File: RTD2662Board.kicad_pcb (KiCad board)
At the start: 2 copper layers, 100 x 65 mm, 227 parts, among them J1 USB_B, J10 Conn_Coaxial, J11 Conn_01x03, J2 AudioJack4, J3 Jack, J4 Conn_02x25_Odd_Even, J5 AudioJack4, J6 DVI_FEMALE, J7 HDMI_A_1.4, J8 Mini-DIN-4, J9 DB15_Female_HighDensity_Mount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, Q5 BC846, Q7 AO3401A, Q8 BC846, Q9 BC846, SW1 SW_Push, SW2 SW_Push, SW3 SW_Push, SW4 SW_Push, SW5 SW_Push, U1 TSOP382xx, U10 TPS61040DBV, U11 TPS61040DBV, U12 CH341T, U2 ES7134S, U4 PAM8003, U5 TPS61040DBV, U6 APW7313, U7 AMS1117-1.8, U8 RTD2662, U9 W25Qxx, Y1 Crystal, Y2 Crystal

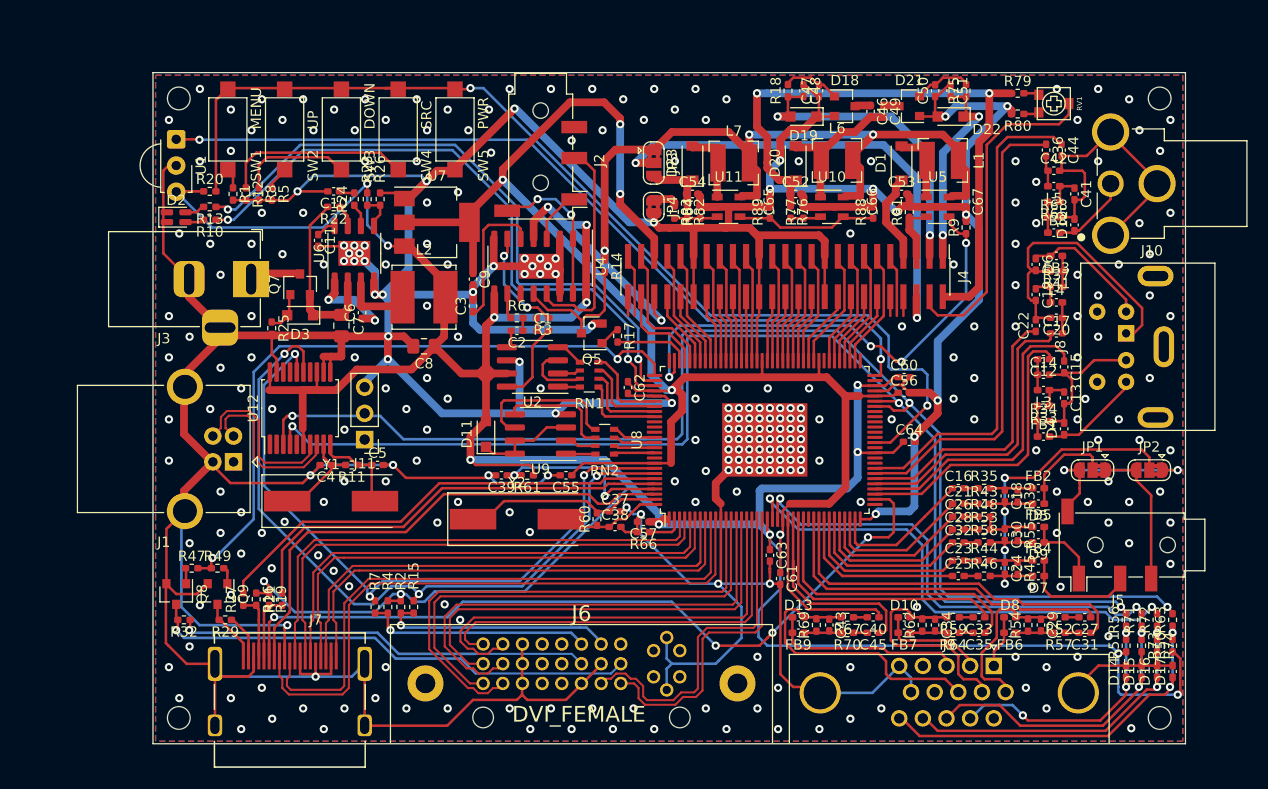
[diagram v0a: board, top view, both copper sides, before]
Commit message: Revision 0.2
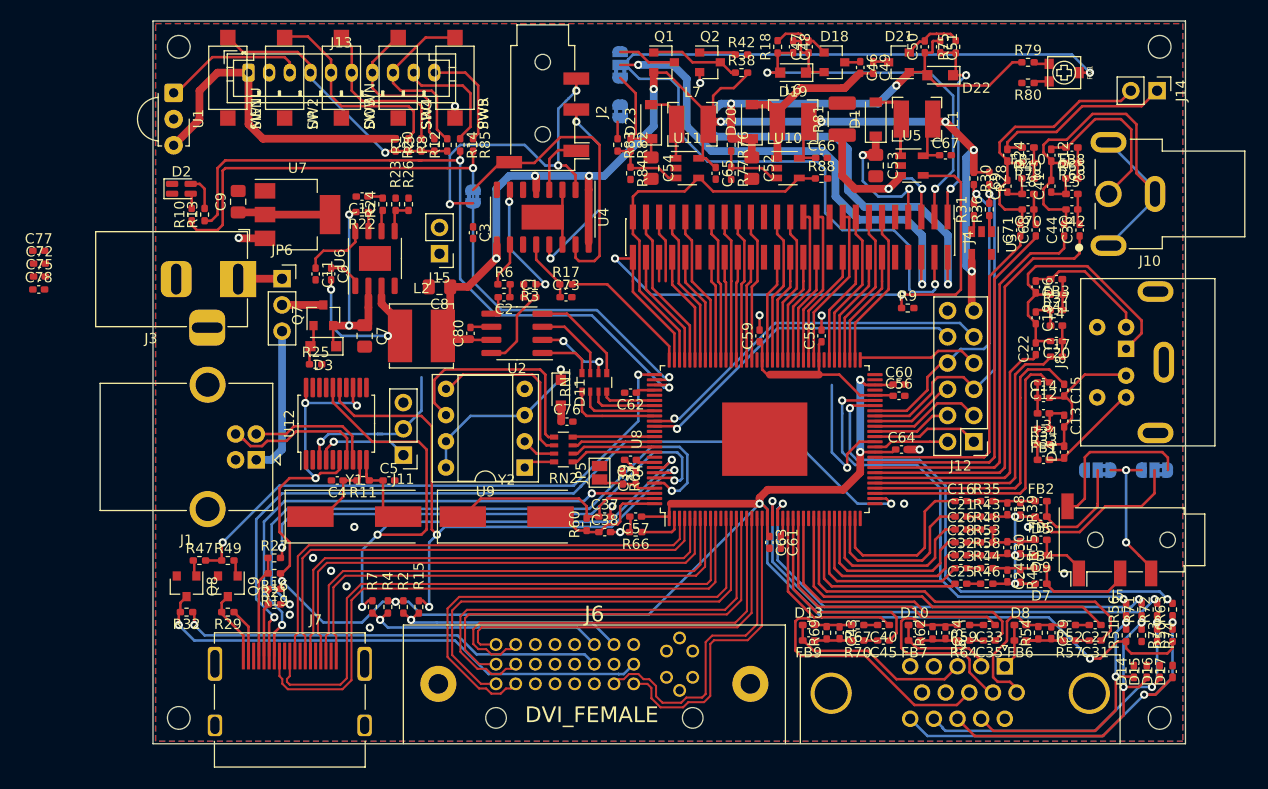
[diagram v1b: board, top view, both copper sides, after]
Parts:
- removed Q5: BC846, Package_TO_SOT_SMD:SOT-23
- removed R89: R, Resistor_SMD:R_0402_1005Metric_Pad0.72x0.64mm_HandSolder
- added C58: C, Capacitor_SMD:C_0402_1005Metric_Pad0.74x0.62mm_HandSolder, F.Cu at (112.2, 105.5)
- added C59: C, Capacitor_SMD:C_0402_1005Metric_Pad0.74x0.62mm_HandSolder, F.Cu at (106.2, 105.5)
- added C68: C, Capacitor_SMD:C_0402_1005Metric_Pad0.74x0.62mm_HandSolder, F.Cu at (133.0, 95.2)
- added C69: C, Capacitor_SMD:C_0402_1005Metric_Pad0.74x0.62mm_HandSolder, F.Cu at (130.2, 91.0)
- added C70: C, Capacitor_SMD:C_0402_1005Metric_Pad0.74x0.62mm_HandSolder, F.Cu at (132.2, 93.2)
- added C71: C, Capacitor_SMD:C_0402_1005Metric_Pad0.74x0.62mm_HandSolder, F.Cu at (131.5, 95.2)
- added C72: C, Capacitor_SMD:C_0402_1005Metric_Pad0.74x0.62mm_HandSolder, F.Cu at (36.5, 98.5)
- added C73: C, Capacitor_SMD:C_0402_1005Metric_Pad0.74x0.62mm_HandSolder, F.Cu at (87.5, 101.8)
- added C75: C, Capacitor_SMD:C_0402_1005Metric_Pad0.74x0.62mm_HandSolder, F.Cu at (36.5, 99.8)
- added C76: C, Capacitor_SMD:C_0402_1005Metric_Pad0.74x0.62mm_HandSolder, F.Cu at (87.6, 113.8)
- added C77: C, Capacitor_SMD:C_0402_1005Metric_Pad0.74x0.62mm_HandSolder, F.Cu at (36.4, 97.2)
- added C78: C, Capacitor_SMD:C_0402_1005Metric_Pad0.74x0.62mm_HandSolder, F.Cu at (36.4, 101.0)
- added C80: C, Capacitor_SMD:C_0402_1005Metric_Pad0.74x0.62mm_HandSolder, F.Cu at (78.2, 105.2)
- added D24: D_TVS, Inductor_SMD:L_0402_1005Metric_Pad0.77x0.64mm_HandSolder, F.Cu at (130.2, 88.0)
- added FB10: 120Ω, Inductor_SMD:L_0402_1005Metric_Pad0.77x0.64mm_HandSolder, F.Cu at (132.2, 87.2)
- added J12: Conn_02x06_Odd_Even, Connector_PinHeader_2.54mm:PinHeader_2x06_P2.54mm_Vertical, F.Cu at (127.0, 115.8)
- added J13: Conn_01x10, Connector_JST:JST_PH_B10B-PH-K_1x10_P2.00mm_Vertical, F.Cu at (56.8, 80.0)
- added J14: Conn_01x02, Connector_PinHeader_2.54mm:PinHeader_1x02_P2.54mm_Vertical, F.Cu at (144.8, 81.8)
- added J15: Conn_01x02, Connector_PinHeader_2.54mm:PinHeader_1x02_P2.54mm_Vertical, F.Cu at (75.2, 97.5)
- added JP5: Reset Pad, Jumper:SolderJumper-2_P1.3mm_Open_Pad1.0x1.5mm, F.Cu at (90.8, 118.8)
- added JP6: Power select, Connector_PinSocket_2.54mm:PinSocket_1x03_P2.54mm_Vertical, F.Cu at (60.0, 100.0)
- added JP7: Jump, Jumper:SolderJumper-2_P1.3mm_Bridged2Bar_RoundedPad1.0x1.5mm, B.Cu at (78.5, 92.0)
- added L8: L, Inductor_SMD:L_0402_1005Metric_Pad0.77x0.64mm_HandSolder, F.Cu at (132.2, 91.8)
- added Q1: AO3401A, Package_TO_SOT_SMD:SOT-23, F.Cu at (97.0, 79.0)
- added Q2: BC846, Package_TO_SOT_SMD:SOT-23, F.Cu at (101.5, 79.0)
- added R28: R, Resistor_SMD:R_0402_1005Metric_Pad0.72x0.64mm_HandSolder, F.Cu at (128.5, 90.2)
- added R30: R, Resistor_SMD:R_0402_1005Metric_Pad0.72x0.64mm_HandSolder, F.Cu at (127.0, 90.2)
- added R31: R, Resistor_SMD:R_0402_1005Metric_Pad0.72x0.64mm_HandSolder, F.Cu at (127.0, 93.2)
- added R36: R, Resistor_SMD:R_0402_1005Metric_Pad0.72x0.64mm_HandSolder, F.Cu at (128.5, 93.2)
- added R38: R, Resistor_SMD:R_0402_1005Metric_Pad0.72x0.64mm_HandSolder, F.Cu at (104.5, 80.0)
- added R40: R, Resistor_SMD:R_0402_1005Metric_Pad0.72x0.64mm_HandSolder, F.Cu at (132.2, 90.2)
- added R42: R, Resistor_SMD:R_0402_1005Metric_Pad0.72x0.64mm_HandSolder, F.Cu at (104.5, 78.2)
- added R78: 75Ω, Resistor_SMD:R_0402_1005Metric_Pad0.72x0.64mm_HandSolder, F.Cu at (132.2, 88.8)
- added R85: R, Resistor_SMD:R_0402_1005Metric_Pad0.72x0.64mm_HandSolder, F.Cu at (78.5, 87.0)
- added U3: AT24CS08-STUM, Package_TO_SOT_SMD:SOT-23-5, F.Cu at (127.8, 96.5)
- C52, C53, C54, C9: footprint Capacitor_SMD:C_0402_1005Metric_Pad0.74x0.62mm_HandSolder -> Capacitor_SMD:C_0805_2012Metric_Pad1.18x1.45mm_HandSolder
- JP1, JP2, JP3, JP4: moved to B.Cu
- R81: footprint Resistor_SMD:R_0402_1005Metric_Pad0.72x0.64mm_HandSolder -> Resistor_SMD:R_1210_3225Metric_Pad1.30x2.65mm_HandSolder
- SW1: value SW_Push -> POWER
- SW2: value SW_Push -> MENU
- SW3: value SW_Push -> UP
- SW4: value SW_Push -> DOWN
- SW5: value SW_Push -> SOURCE
- U9: footprint Package_SO:SOIC-8_3.9x4.9mm_P1.27mm -> Package_DIP:DIP-8_W7.62mm_Socket
- moved C9 24.0 mm to (55.8, 92.5), turned to 90 degrees
- moved R12 20.1 mm to (76.0, 87.0), turned to 90 degrees
- moved R20 18.6 mm to (71.0, 87.0), turned to 270 degrees
- moved R14 18.3 mm to (77.2, 87.0)
- moved R1 17.7 mm to (72.2, 87.0), turned to 90 degrees
- moved R8 17.7 mm to (74.8, 87.0), turned to 90 degrees
- moved R5 15.3 mm to (73.5, 87.0), turned to 90 degrees
- moved U7 13.5 mm to (61.5, 93.8)
- moved C39 13.0 mm to (94.2, 119.2), turned to 90 degrees
- moved R81 11.1 mm to (114.2, 84.5)
- moved JP3 10.0 mm to (92.8, 79.2), turned to 90 degrees
- moved JP4 9.80 mm to (92.8, 83.8)
- moved R9 9.63 mm to (120.6, 102.8), turned to 0 degrees
- moved R61 9.25 mm to (93.0, 119.2), turned to 270 degrees
- moved R76 8.68 mm to (103.5, 87.0)
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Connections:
- net CVBS+ renamed CVBS0+
- net CVBS- renamed CVBS0-
- net I2S_SDAT renamed I2S_SDAT0
- net Net-(U8-Pad114) renamed I2S_SDAT3
- net _CVBS+ renamed _CVBS0+
- net _CVBS- renamed _CVBS0-
- C50 pad 1: GND -> AVCC
- C51 pad 1: GND -> AVCC
- D21 pad 1: GND -> AVCC
- D22 pad 2: GND -> AVCC
- J1 pad 1: Net-(J1-Pad1) -> VUSB
- J4 pad 49: Net-(J4-Pad49) -> EN_LCD
- J4 pad 50: Net-(J4-Pad50) -> EN_BL
- JP3 pad 1: +3V3 -> Net-(JP3-Pad1)
- Q7 pad 3: Net-(J3-Pad1) -> Net-(JP6-Pad2)
- R1 pad 1: Net-(R1-Pad1) -> BUTTONS
- R1 pad 2: GND -> MENUB
- R10 pad 1: RED_LED -> GRN_LED
- R12 pad 1: Net-(R12-Pad1) -> BUTTONS
- R12 pad 2: GND -> SRCB
- R13 pad 1: GRN_LED -> RED_LED
- R14 pad 1: +3V3 -> Net-(J13-Pad9)
- R14 pad 2: Net-(Q5-Pad3) -> RED_LED
- R17 pad 1: Net-(Q5-Pad1) -> Net-(C73-Pad1)
- R5 pad 1: Net-(R5-Pad1) -> BUTTONS
- R5 pad 2: GND -> UPB
- R8 pad 1: Net-(R8-Pad1) -> BUTTONS
- R8 pad 2: GND -> DWNB
- R88 pad 1: EN_REF -> EN_LCD
- SW1 pad 1: Net-(R1-Pad1) -> GND
- SW2 pad 1: Net-(R5-Pad1) -> GND
- SW2 pad 2: BUTTONS -> MENUB
- SW3 pad 1: Net-(R8-Pad1) -> GND
- SW3 pad 2: BUTTONS -> UPB
- SW4 pad 1: Net-(R12-Pad1) -> GND
- SW4 pad 2: BUTTONS -> DWNB
- SW5 pad 2: BUTTONS -> SRCB
- U10 pad 4: EN_REF -> EN_LCD
- U11 pad 4: EN_REF -> EN_LCD
- U4 pad 12: Net-(Q5-Pad3) -> Net-(C73-Pad1)
- U4 pad 2: Net-(J2-PadS) -> Net-(J2-PadR2)
- U8 pad 100: VOL -> EN_LCD
- U8 pad 102: Net-(U8-Pad102) -> VOL
- U8 pad 112: Net-(U8-Pad112) -> I2S_SDAT1
- U8 pad 113: Net-(U8-Pad113) -> I2S_SDAT2
- U8 pad 47: Net-(U8-Pad47) -> CVBS1+
- U8 pad 48: Net-(U8-Pad48) -> CVBS1-
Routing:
- net GND: track 682.3 -> 26.4 mm, vias 308 -> 16
- net +1V8: track 146.8 -> 41.3 mm, vias 5 -> 0
- net IRDA: track 79.7 -> 13.9 mm, vias 2 -> 0
- net VCOM: track 32.3 -> 97.2 mm, vias 0 -> 2
- net BUTTONS: track 102.6 -> 39.7 mm
- net TX: track 116.2 -> 56.6 mm
- net RX: track 124.3 -> 65.4 mm
- net +3V3: track 398.9 -> 358.7 mm
- net EN_LCD: track 0.00 -> 36.9 mm
- net I2S_SDAT1: track 0.00 -> 35.5 mm, vias 0 -> 1
- net CVBS1+: track 0.00 -> 34.9 mm
- net EIO6: track 0.00 -> 34.0 mm, vias 0 -> 1
- net CVBS1-: track 0.00 -> 33.5 mm
- net I2S_SDAT2: track 0.00 -> 33.0 mm, vias 0 -> 1
- net EIO7: track 0.00 -> 31.4 mm, vias 0 -> 1
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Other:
- board size 100 x 65 mm -> 100 x 70 mm
- net class LCD Signal removed
- net class Power added: clearance 0.2, trace_width 0.75, via_dia 0.8, via_drill 0.4

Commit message: Revision 1.0
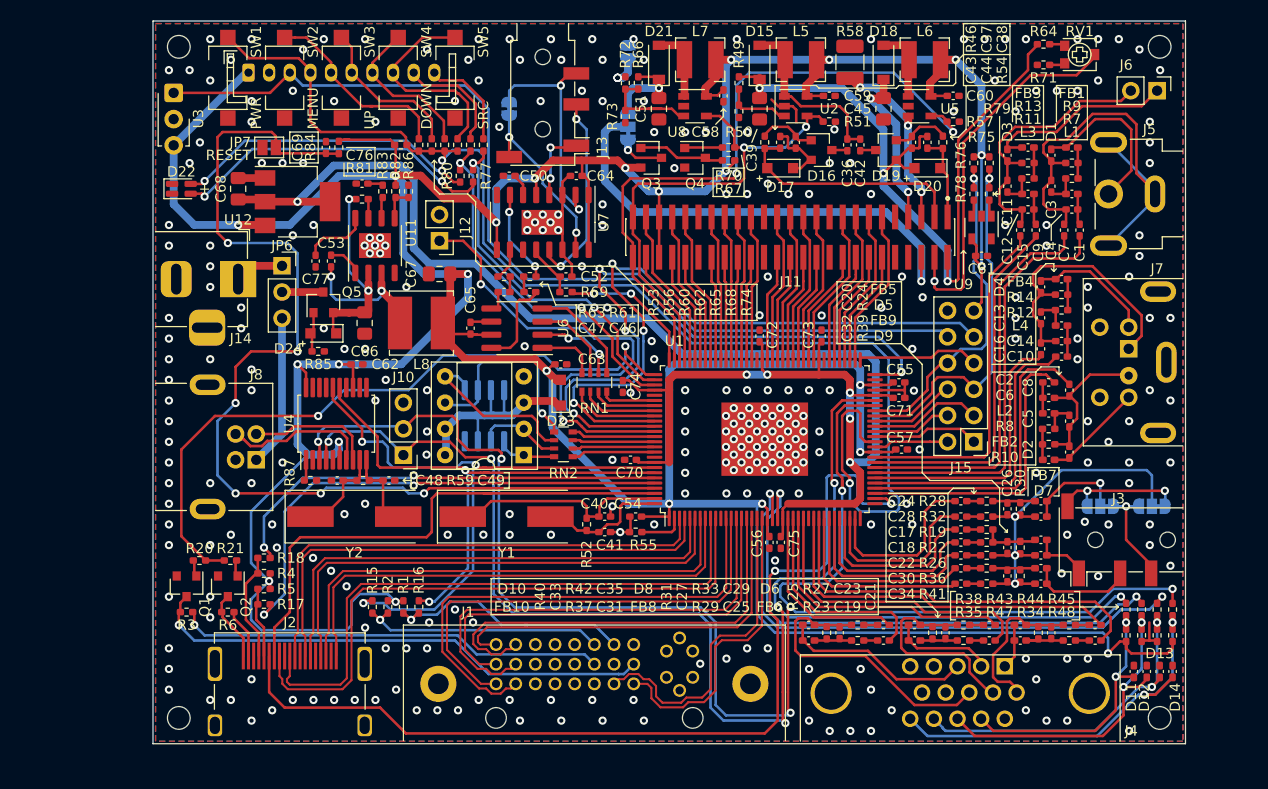
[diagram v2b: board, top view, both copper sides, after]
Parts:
- removed C78, C80: C, Capacitor_SMD:C_0402_1005Metric_Pad0.74x0.62mm_HandSolder
- removed the J6 at (90.2, 142.5)
- removed the R9 at (120.6, 102.8)
- removed the U9 at (83.5, 118.2)
- added C65: C, Capacitor_SMD:C_0402_1005Metric_Pad0.74x0.62mm_HandSolder, F.Cu at (78.2, 104.8)
- added J1: DVI_Female, RTD2662Board:DVI, F.Cu at (90.2, 142.5)
- added R57: R, Resistor_SMD:R_0402_1005Metric_Pad0.72x0.64mm_HandSolder, F.Cu at (125.0, 84.8)
- added R87: R, Resistor_SMD:R_0402_1005Metric_Pad0.72x0.64mm_HandSolder, F.Cu at (62.8, 119.5)
- added U10: W25Qxx, RTD2662Board:SOIC-8_3.9x4.9mm_P1.27mm_DIP-8_W7.62mm_Socket, F.Cu at (79.6, 113.2)
- D22: renamed from D2; value LED_Dual_ACAC -> Dual LED
- J10: renamed from J11; value Conn_01x03 -> UART/I2C
- J11: renamed from J4; value Conn_02x25_Odd_Even -> LCD Connector
- J12: renamed from J15; value Conn_01x02 -> SPDIFF
- J15: renamed from J12; value Conn_02x06_Odd_Even -> Expansion Connector
- J9: renamed from J13; value Conn_01x10 -> Keyboard Connector
- JP4: footprint Jumper:SolderJumper-2_P1.3mm_Bridged2Bar_RoundedPad1.0x1.5mm -> Jumper:SolderJumper-2_P1.3mm_Open_RoundedPad1.0x1.5mm
- moved C61 91.3 mm to (127.8, 97.8)
- moved C64 52.6 mm to (88.5, 90.0), turned to 180 degrees
- moved JP7 44.9 mm to (58.8, 87.2), turned to 180 degrees
- moved C69 43.9 mm to (64.2, 87.2)
- moved R84 42.2 mm to (65.5, 87.2)
- moved C62 31.9 mm to (67.2, 108.2)
- moved R77 27.5 mm to (78.5, 90.0), turned to 270 degrees
- moved R80 25.0 mm to (77.2, 90.0), turned to 270 degrees
- moved REF** 13.5 mm to (52.8, 96.2)
- moved Q4 9.36 mm to (100.0, 88.2)
- moved C37 9.33 mm to (109.8, 86.8)
- moved C38 9.33 mm to (108.2, 86.8)
- moved C43 9.33 mm to (121.0, 86.8)
- moved C44 9.33 mm to (122.5, 86.8)
- moved D17 9.33 mm to (108.2, 89.2)
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- renumbered C36 to C1, C17 to C10, C69 to C11, C70 to C12, C19 to C13, C20 to C14, C71 to C15, C22 to C16, C26 to C17, C28 to C18, C31 to C19, C12 to C2, C30 to C20, C29 to C21, C32 to C22, C27 to C23, C16 to C24, C35 to C25, C18 to C26, C34 to C27, C21 to C28, C33 to C29, C41 to C3, C23 to C30, C45 to C31, C24 to C32, C43 to C33, C25 to C34, C40 to C35, C46 to C36, C47 to C37, C48 to C38, C52 to C39, C42 to C4, C37 to C40, C38 to C41, C49 to C42, C50 to C43, C51 to C44, C53 to C45, C1 to C46, C2 to C47, C4 to C48, C5 to C49, C13 to C5, C3 to C50, C54 to C51, C73 to C52, C6 to C53, C57 to C54, C60 to C55, C63 to C56, C64 to C57, C65 to C58, C66 to C59, C14 to C6, C67 to C60, C72 to C61, C75 to C62, C76 to C63, C77 to C64, C7 to C66, C8 to C67, C9 to C68, C39 to C69, C44 to C7, C55 to C70, C56 to C71, C59 to C72, C58 to C73, C62 to C74, C61 to C75, C10 to C76, C11 to C77, C15 to C8, C68 to C9, D12 to D1, D13 to D10, D14 to D11, D15 to D12, D16 to D13, D17 to D14, D20 to D15, D18 to D16, D19 to D17, D1 to D18, D21 to D19, D4 to D2, D22 to D20, D23 to D21, D11 to D23, D3 to D24, D24 to D3, D6 to D4, D9 to D5, D8 to D6, D5 to D7, D10 to D8, D7 to D9, FB8 to FB1, FB9 to FB10, FB1 to FB2, FB10 to FB3, FB3 to FB4, FB2 to FB7, FB7 to FB8, FB4 to FB9, J2 to J13, J3 to J14, J7 to J2, J5 to J3, J9 to J4, J10 to J5, J14 to J6, J8 to J7, J1 to J8, JP7 to JP5, JP5 to JP7, L5 to L1, L3 to L2, L8 to L3, L6 to L5, L1 to L6, L2 to L8, Q8 to Q1, Q9 to Q2, Q1 to Q3, Q2 to Q4, Q7 to Q5, R2 to R1, R34 to R10, R40 to R11, R37 to R12, R78 to R13, R41 to R14, R7 to R15, R15 to R16, R21 to R17, R27 to R18, R48 to R19, R4 to R2, R47 to R20, R49 to R21, R53 to R22, R57 to R23, R55 to R24, R54 to R25, R58 to R26, R52 to R27, R35 to R28, R64 to R29, R32 to R3, R39 to R30, R62 to R31, R43 to R32, R59 to R33, R50 to R34, R51 to R35, R44 to R36, R70 to R37, R56 to R38, R45 to R39, R16 to R4, R69 to R40, R46 to R41, R67 to R42, R71 to R43, R72 to R44, R63 to R45, R18 to R46, R73 to R47, R74 to R48, R76 to R49, R19 to R5, R77 to R50, R88 to R51, R60 to R52, R20 to R53, R75 to R54, R66 to R55, R1 to R56, R81 to R58, R11 to R59, R29 to R6, R5 to R60, R3 to R61, R8 to R62, R6 to R63, R79 to R64, R12 to R65, R82 to R66, R38 to R67, R14 to R68, R17 to R69, R65 to R7, R42 to R70, R80 to R71, R83 to R72, R84 to R73, R85 to R74, R28 to R75, R30 to R76, R10 to R77, R31 to R78, R36 to R79, R33 to R8, R13 to R80, R22 to R81, R23 to R82, R24 to R83, R61 to R84, R25 to R85, R26 to R86, R68 to R9, U8 to U1, U6 to U11, U7 to U12, U10 to U2, U1 to U3, U12 to U4, U2 to U6, U4 to U7, U11 to U8, U3 to U9, Y2 to Y1, Y1 to Y2
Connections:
- net Net-(C39-Pad1) renamed ~RESET~
- net Net-(J2-PadR1) renamed RIGHT+
- net Net-(J2-PadR2) renamed LEFT-
- net Net-(J2-PadS) renamed RIGHT-
- net Net-(J2-PadT) renamed LEFT+
- C11 pad 2: _CVBS1- -> GND
- C12 pad 2: _CVBS1- -> GND
- C13 pad 2: _S_Y- -> GND
- C14 pad 2: _S_Y- -> GND
- C15 pad 2: _CVBS1- -> GND
- C16 pad 2: _S_Y- -> GND
- C20 pad 2: _B_Pb- -> GND
- C21 pad 1: _VGA_R- -> GND
- C26 pad 2: _B_Pb- -> GND
- C27 pad 1: _VGA_G- -> GND
- C3 pad 2: _CVBS0- -> GND
- C32 pad 2: _B_Pb- -> GND
- C33 pad 1: _VGA_B- -> GND
- C4 pad 2: _CVBS0- -> GND
- C5 pad 2: _S_C- -> GND
- C6 pad 2: _S_C- -> GND
- C7 pad 2: _CVBS0- -> GND
- C8 pad 2: _S_C- -> GND
- D1 pad 2: _CVBS0- -> GND
- D10 pad 2: _VGA_B- -> GND
- D2 pad 2: _S_C- -> GND
- D3 pad 2: _CVBS1- -> GND
- D4 pad 2: _S_Y- -> GND
- D5 pad 2: _B_Pb- -> GND
- D6 pad 2: _VGA_R- -> GND
- D7 pad 2: _B_Pb- -> GND
- D8 pad 2: _VGA_G- -> GND
- D9 pad 2: _B_Pb- -> GND
- J11 pad 45: +1V8 -> +3V3
- J12 pad 1: I2S_SDAT1 -> I2S_SDAT3
- J4 pad 6: _VGA_R- -> GND
- J4 pad 7: _VGA_G- -> GND
- J4 pad 8: _VGA_B- -> GND
- J5 pad 2: _CVBS0- -> GND
- J6 pad 2: _CVBS1- -> GND
- J7 pad 1: _S_Y- -> GND
- J7 pad 2: _S_C- -> GND
- JP2 pad 2: _B_Pb- -> GND
- R10 pad 2: _S_C- -> GND
- R13 pad 2: _CVBS1- -> GND
- R14 pad 2: _S_Y- -> GND
- R24 pad 2: _B_Pb- -> GND
- R25 pad 2: _VGA_R- -> GND
- R26 pad 2: _B_Pb- -> GND
- R27 pad 2: _VGA_R- -> GND
- R30 pad 2: _B_Pb- -> GND
- R31 pad 2: _VGA_G- -> GND
- R32 pad 2: _B_Pb- -> GND
- R33 pad 2: _VGA_G- -> GND
- R39 pad 2: _B_Pb- -> GND
- R40 pad 2: _VGA_B- -> GND
- R41 pad 2: _B_Pb- -> GND
- R42 pad 2: _VGA_B- -> GND
- R9 pad 2: _CVBS0- -> GND
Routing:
- net GND: track 26.4 -> 248.4 mm, vias 16 -> 320
- net +1V8: track 41.3 -> 158.5 mm, vias 0 -> 6
- net +3V3: track 358.7 -> 461.7 mm, vias 19 -> 24
- net ~RESET~: track 4.86 -> 102.2 mm, vias 0 -> 6
- net TX: track 56.6 -> 147.5 mm, vias 3 -> 6
- net RX: track 65.4 -> 154.4 mm, vias 3 -> 6
- net BUTTONS: track 39.7 -> 123.4 mm
- net IRDA: track 13.9 -> 94.2 mm, vias 0 -> 1
- net VCOM: track 97.2 -> 36.3 mm, vias 2 -> 1
- net I2S_SDAT3: track 0.00 -> 47.0 mm, vias 0 -> 2
- net _CVBS0-: track 42.5 -> 0.00 mm
- net _B_Pb-: track 36.0 -> 0.00 mm, vias 3 -> 0
- net GRN_LED: track 70.4 -> 34.6 mm
- net I2S_SDAT2: track 33.0 -> 67.2 mm, vias 1 -> 3
- net RED_LED: track 68.7 -> 35.2 mm
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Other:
- rule pad_to_mask_clearance: 0 -> 0.05
- board text added: "+3.3V"
- board text added: "1-2 - 3.3V 3-2 - 12V/5V"
- board text added: "AUDIO"
- board text added: "AVCC"
- board text added: "B1/B7/O3+"
- board text added: "B2"
- board text added: "B3"
- board text added: "B4"
- board text added: "B5"
- board text added: "B6"
- board text added: "B7"
- board text added: "BL_ANO"
- board text added: "BL_CAT"
- board text added: "CVBS1"
- board text added: "CVBS2+"
- board text added: "CVBS2-"
- board text added: "DCK"
- board text added: "DEN/E0+"
- board text added: "DVCC"
- board text added: "DVI"
- board text added: "DVS"
- board text added: "E0-/DHS"
- board text added: "E1-/R2/R0"
- board text added: "E2-/R4/R2"
- board text added: "E3-/G2/R6"
- board text added: "EC-/R6/R4"
- board text added: "EN_BL"
- board text added: "EN_LCD"
- board text added: "G1/G5/E0+"
- board text added: "G3/G7/O1+"
- board text added: "G5/B3/O2+"
- board text added: "G7/B5/OC+"
- board text added: "GND"
- board text added: "HDMI"
- board text added: "HMIR"
- board text added: "IO0"
- board text added: "IO1"
- board text added: "IO2"
- board text added: "IO3"
- board text added: "IO4"
- board text added: "IO5"
- board text added: "IO6"
- board text added: "IO7"
- board text added: "IO8"
- board text added: "IO9"
- board text added: "IR"
- board text added: "JACK PWR"
- board text added: "JP1 & JP2: 1-2 - GND-SLEEVE 3-2 - GND-RING2"
- board text added: "LEDA1"
- board text added: "LEDA2"
- board text added: "O-5V C-12V"
- board text added: "O0-/G4/G0"
- board text added: "O1-/G6/G2"
- board text added: "O2-/B2/G4"
- board text added: "O3-/B6/B0"
- board text added: "OC-/B4/G6"
- board text added: "ORTD2662-PROTOBOARD-REV1"
- board text added: "R1/R3/E1+"
- board text added: "R3/R5/E2+"
- board text added: "R5/R7/EC+"
- board text added: "R7/G3/E3+"
- board text added: "RESET"
- board text added: "RGsB YPbPr"
- board text added: "RX/SCL"
- board text added: "S/PDIF"
- board text added: "SVIDEO"
- board text added: "TX/SDA"
- board text added: "USB PWR"
- board text added: "VCOM"
- board text added: "VGA"
- board text added: "VGH"
- board text added: "VGL"
- board text added: "VMIR"
